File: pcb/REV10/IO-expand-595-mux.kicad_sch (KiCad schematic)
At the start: 53 parts, among them Q300 SI2301, Q301 SI2301, Q302 SI2301, Q303 SI2301, Q304 SI2301, Q305 SI2301, Q306 SI2301, Q307 SI2301, U402 CD4067, U404 LMV321, U501 74HC595, U502 74HC595, U503 74HCT245PW, U504 LMV324, U505 LMV324, U506 LMV321

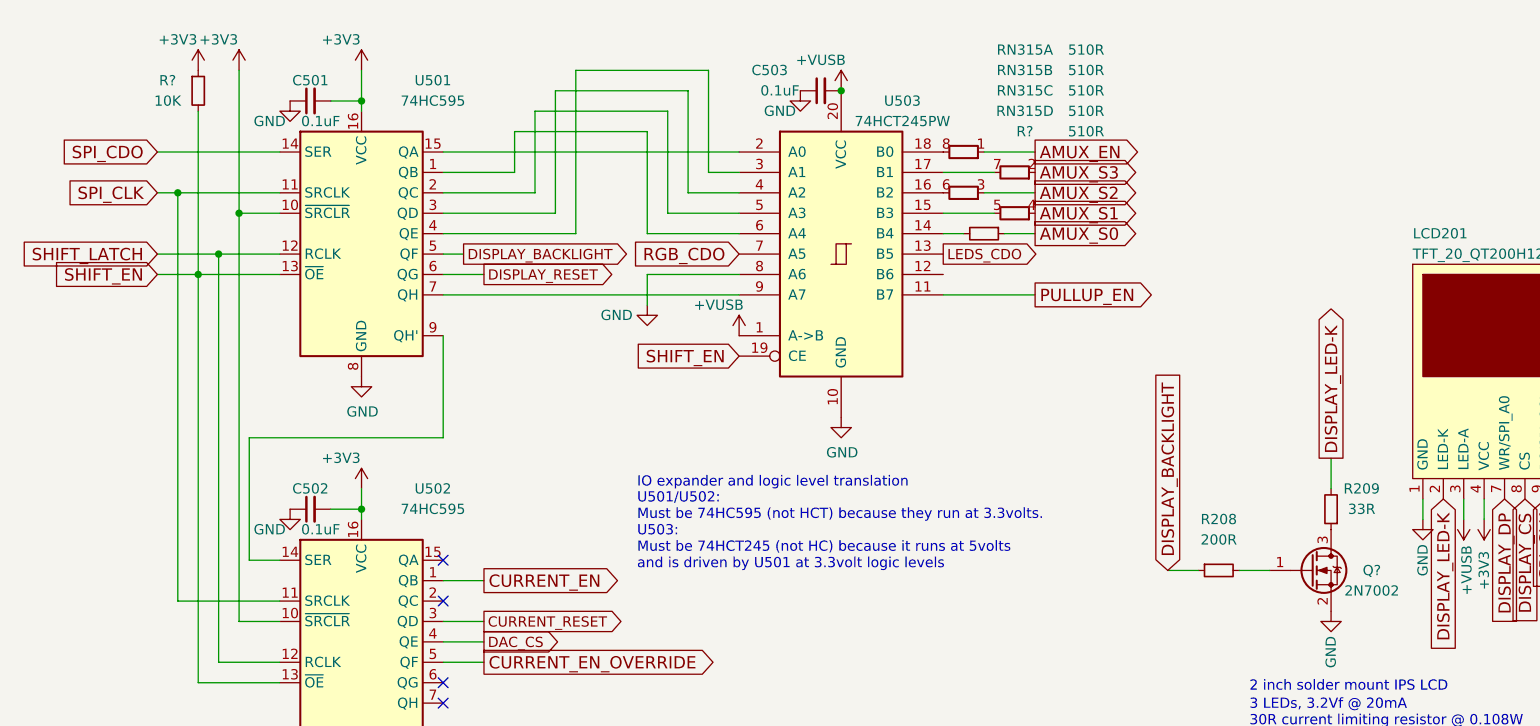
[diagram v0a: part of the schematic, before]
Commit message: making chris branch
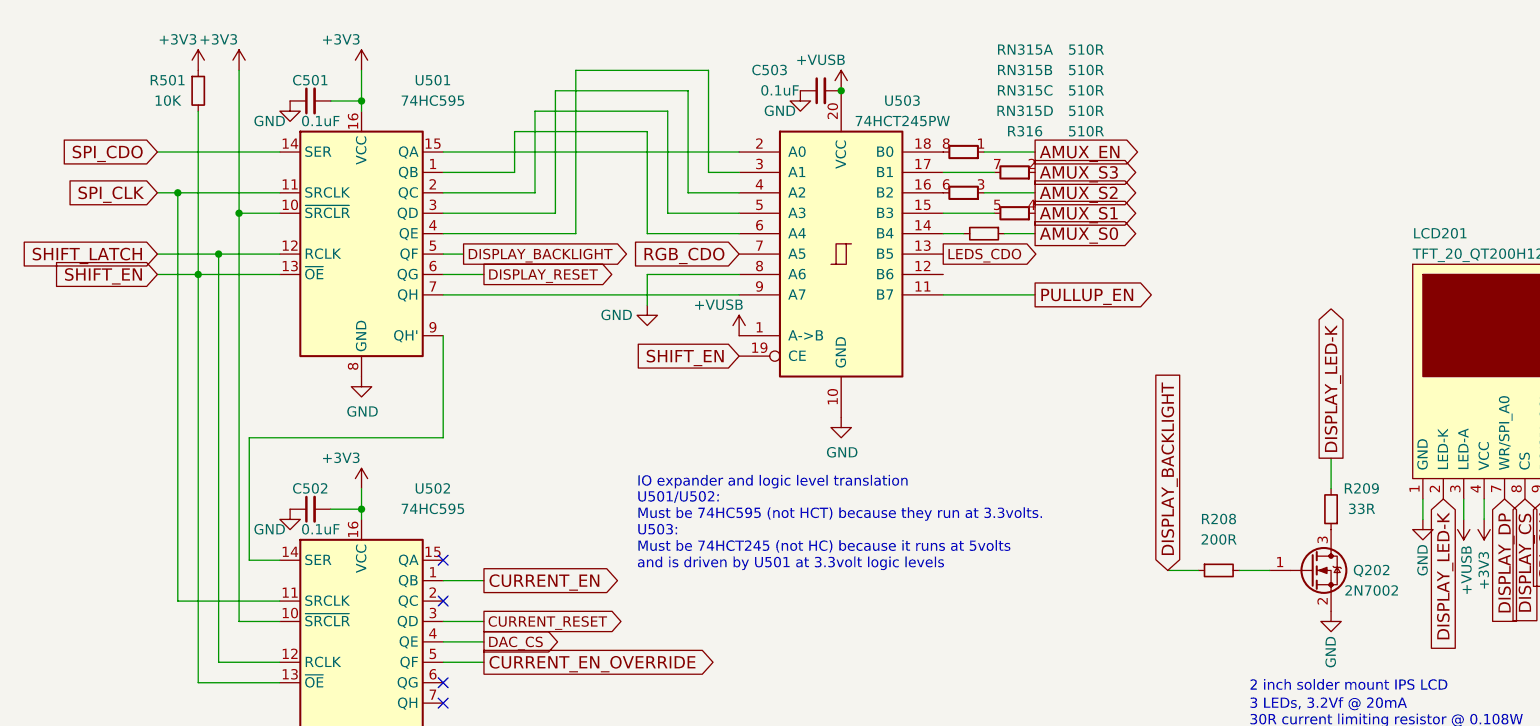
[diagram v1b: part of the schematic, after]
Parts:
- gave numbers to parts that had none: 3

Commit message: clean up directory names
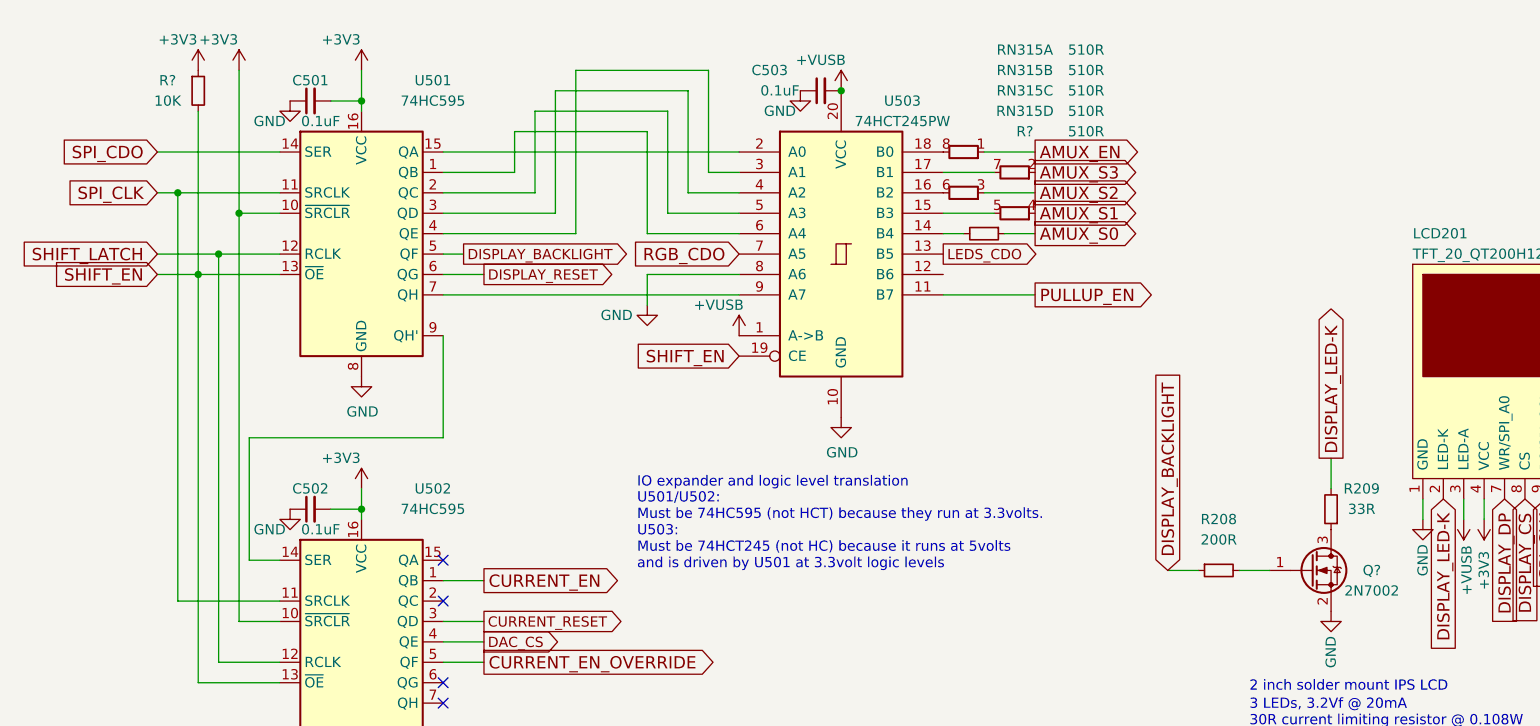
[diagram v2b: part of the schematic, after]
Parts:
- renumbered Q202 to Q?, R501 to R?, R316 to R?
